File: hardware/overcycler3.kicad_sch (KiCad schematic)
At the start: 127 parts, among them J1 USB_B, J2 AudioJack3_Switch, J3 DIN-5_180degree, J4 AudioJack3_Switch, J5 AudioJack3_Switch, P1 FT232, P2 PANEL, Q1 2SC945, SW1 RESET, SW2 POWER, U1 XT26G02CWSIGA, U2 TL074, U20 AD5328B, U3 LPC1778FBD144, U4 TLV2556, U5 74HC138, U6 TL074, U7 AD5328B, Y1 12MHz

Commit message: hardware: adding filters on MIXA/MIXB/MIXN CVs -- needs PCB update
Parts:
- added C112, C113, C114: 100n, Capacitor_SMD:C_0805_2012Metric, symbol overcycler2-rescue:C
- added R93 (x3): 10k, Resistor_SMD:R_0805_2012Metric, symbol overcycler2-rescue:R
- R10: value 27k -> 15k; LCSC C17593 -> C17475
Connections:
- net DAC_MIXA: now also C114.1, R93.1; no longer U20.5 (VOUTB)
- net DAC_MIXB: now also C112.1, R93.1; no longer U20.4 (VOUTA)
- net DAC_MIXN: now also C113.1, R93.1; no longer U7.4 (VOUTA)
- net GND: now also C112.2, C113.2, C114.2
- new net: R93.2, U20.4 (VOUTA)
- new net: R93.2, U7.4 (VOUTA)
- new net: R93.2, U20.5 (VOUTB)
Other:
- moved on the sheet: C38, C39, C40, C41, C42, C43, C44, C45, C46, C47, C49, FB2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

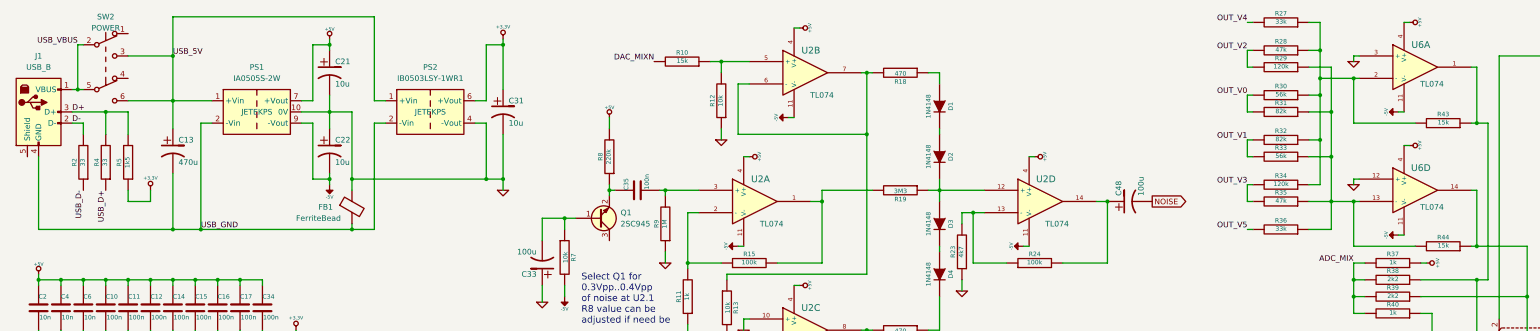
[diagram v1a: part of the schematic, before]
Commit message: hardware: adjusted mixer output level (cf. prev commit), USB ground now entirely disconnected from GND
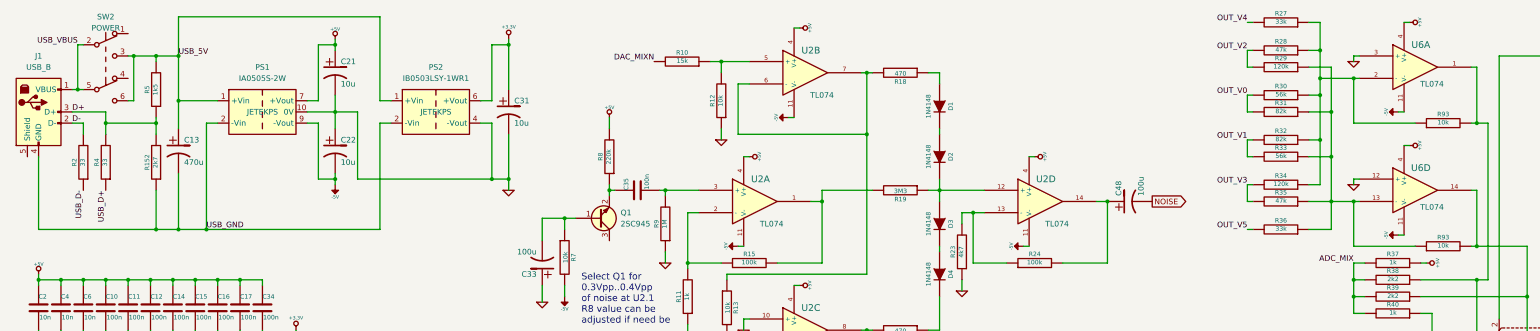
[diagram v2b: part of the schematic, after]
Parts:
- removed FB1: FerriteBead, Inductor_SMD:L_0805_2012Metric, symbol Device:FerriteBead
- removed R43, R44: 15k, Resistor_SMD:R_0805_2012Metric, symbol overcycler2-rescue:R
- added R152: 2k7, Resistor_SMD:R_0805_2012Metric, symbol overcycler2-rescue:R
- added R93 (x2): 10k, Resistor_SMD:R_0805_2012Metric, symbol overcycler2-rescue:R
- C28: LCSC (none) -> C28233
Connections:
- net +3.3V: no longer R5.1
- net D+: now also R5.1, R152.2; no longer R5.2
- net USB_5V: now also R5.2
- net USB_GND: now also R152.1
- net at R29.1, R31.1, R33.1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: now also R93.1
- net at R27.1, R28.1, R30.1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: now also R93.1
- net at R38.1, RV1.1, U6.1: now also R93.2
- net at R39.1, RV1.4, U6.14: now also R93.2
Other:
- moved on the sheet: C13, C21, C22, C31, PS1, PS2
